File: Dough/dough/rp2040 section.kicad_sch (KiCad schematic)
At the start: 71 parts, among them J11 Conn_01x10_Pin, J2 Conn_01x05_Pin, J4 servo 6, J5 servo 1, J6 servo 2, J7 servo 3, J8 servo 4, J9 servo 5, Q2 2N7002, Q5 2N7002, SW1 2040 RST, SW301 2040 BOOTSEL, U1 W25Q32JVSS, U11 25SH-B-04-TS, U2 RP2040, U6 BMP581, U7 MMC5633NJL, U8 BMI160, X1 ECS-2520MV-xxx-xx

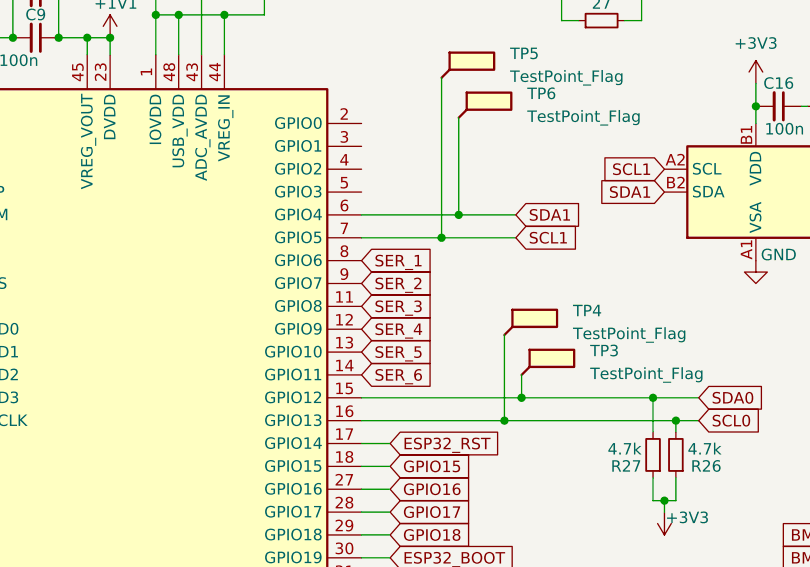
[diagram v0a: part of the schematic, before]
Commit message: dough First production run
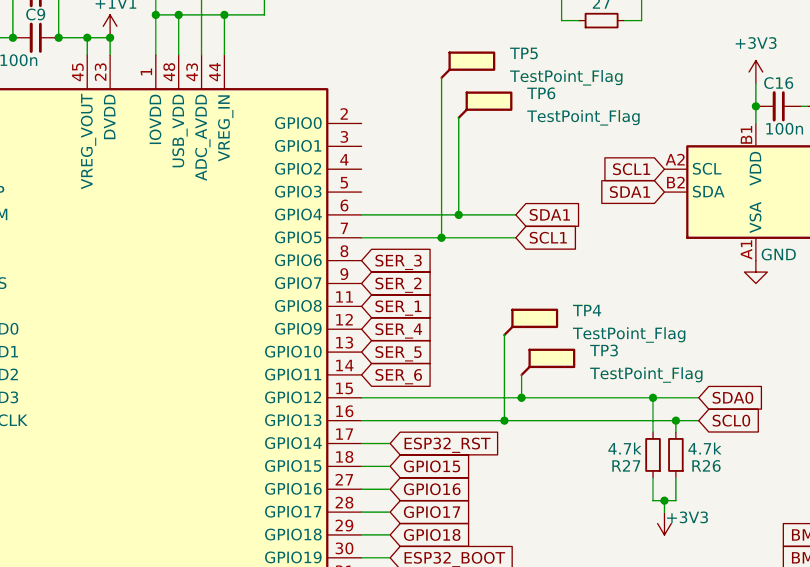
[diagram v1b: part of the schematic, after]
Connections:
- net SER_1: now also U2.11 (GPIO8); no longer U2.8 (GPIO6)
- net SER_3: now also U2.8 (GPIO6); no longer U2.11 (GPIO8)
